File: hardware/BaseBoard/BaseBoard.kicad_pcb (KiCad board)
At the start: 2 copper layers, 81.5 x 109.2 mm, 91 parts, among them J1 I2C, J1-ESP1 ESP-1-L, J1-ESP2 ESP-1-L, J1-ESP3 ESP-1-L, J1-ESP4 ESP-1-L, J1-ESP5 ESP-1-L, J1-ESP6 ESP-1-L, J1-ESP7 ESP-1-L, J1-ESP8 ESP-1-L, J2 3V3P0_7, J2-ESP1 ESP-1-R, J2-ESP2 ESP-1-R, J2-ESP3 ESP-1-R, J2-ESP4 ESP-1-R, J2-ESP5 ESP-1-R, J2-ESP6 ESP-1-R, J2-ESP7 ESP-1-R, J2-ESP8 ESP-1-R, J3-BUS1 BUS1-IN1, J3-BUS2 BUS1-IN1, J3-BUS3 BUS1-IN1, J3-BUS4 BUS1-IN1, J3-BUS5 BUS1-IN1, J3-BUS6 BUS1-IN1, J3-BUS7 BUS1-IN1, J3-BUS8 BUS1-IN1, J4-BUS1 BUS1-IN2, J4-BUS2 BUS1-IN2, J4-BUS3 BUS1-IN2, J4-BUS4 BUS1-IN2, J4-BUS5 BUS1-IN2, J4-BUS6 BUS1-IN2, J4-BUS7 BUS1-IN2, J4-BUS8 BUS1-IN2, J5-BUS1 BUS1-OUT, J5-BUS2 BUS1-OUT, J5-BUS3 BUS1-OUT, J5-BUS4 BUS1-OUT, J5-BUS5 BUS1-OUT, J5-BUS6 BUS1-OUT, J5-BUS7 BUS1-OUT, J5-BUS8 BUS1-OUT, Q1-ESP1 2N3904, Q1-ESP2 2N3904, Q1-ESP3 2N3904, Q1-ESP4 2N3904, Q1-ESP5 2N3904, Q1-ESP6 2N3904, Q1-ESP7 2N3904, Q1-ESP8 2N3904, Q2-ESP1 AO3401A, Q2-ESP2 AO3401A, Q2-ESP3 AO3401A, Q2-ESP4 AO3401A, Q2-ESP5 AO3401A, Q2-ESP6 AO3401A, Q2-ESP7 AO3401A, Q2-ESP8 AO3401A, U1 AMS1117-3.3

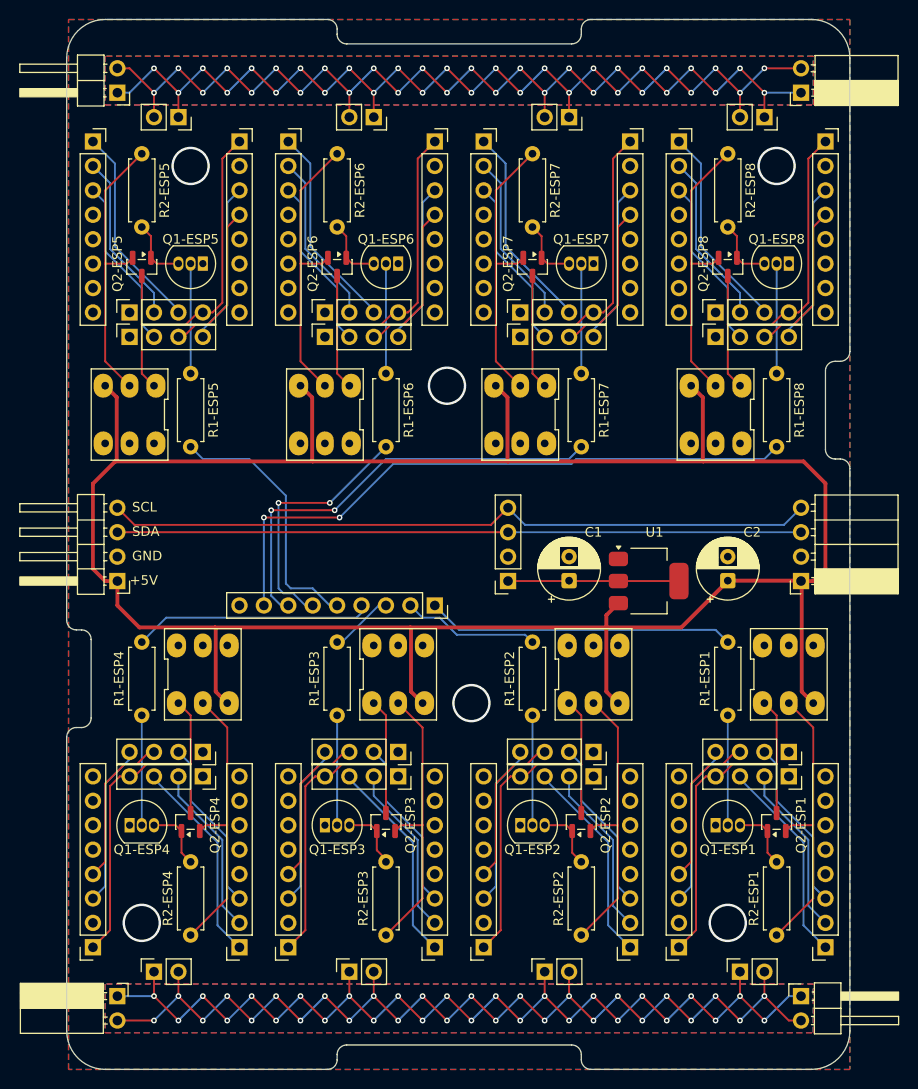
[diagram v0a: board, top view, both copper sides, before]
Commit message: Small optimizations.
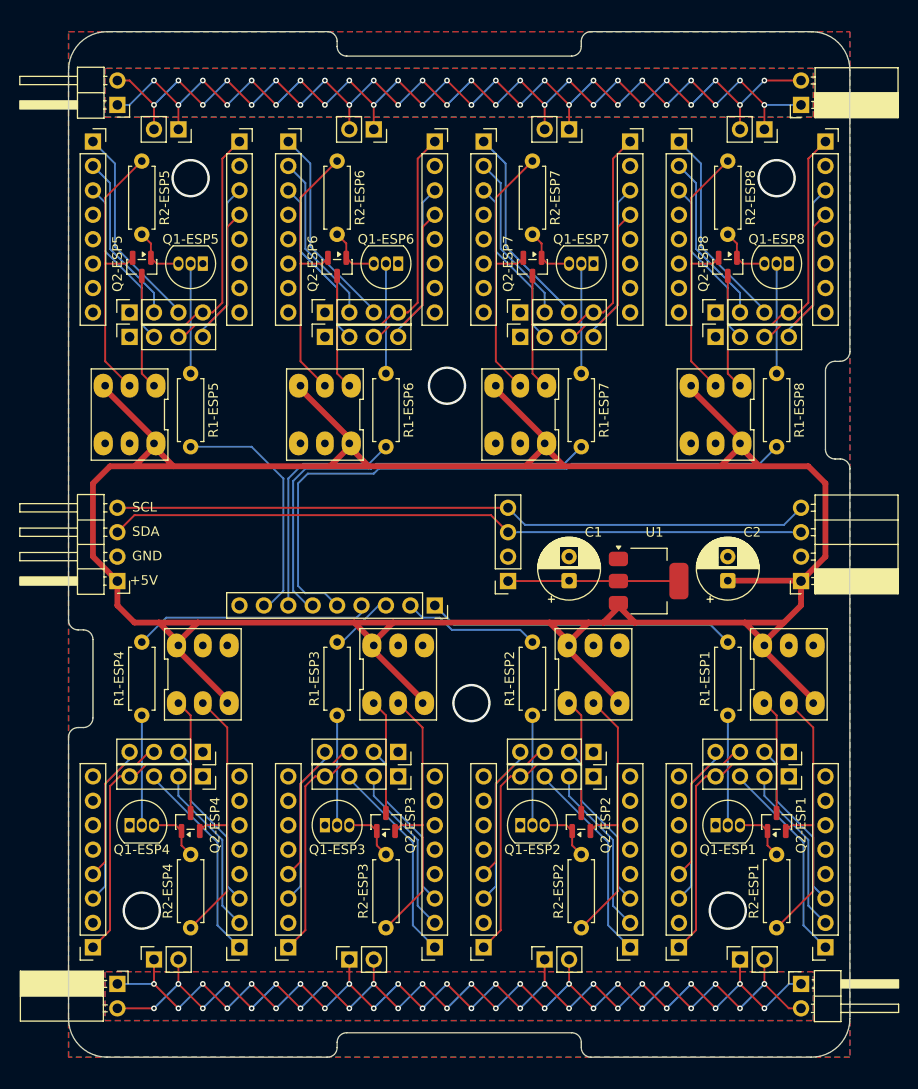
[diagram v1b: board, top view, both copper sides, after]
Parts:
- moved J5-BUS1 1.27 mm to (191.8, 115.6)
- moved J5-BUS2 1.27 mm to (171.4, 115.6)
- moved J5-BUS3 1.27 mm to (151.1, 115.6)
- moved J5-BUS4 1.27 mm to (130.8, 115.6)
- moved BUS_IN2 1.27 mm to (127.0, 26.7)
- moved BUS_OUT2 1.27 mm to (198.1, 26.7)
- moved J5-BUS5 1.27 mm to (133.3, 29.2)
- moved J5-BUS6 1.27 mm to (153.7, 29.2)
- moved J5-BUS7 1.27 mm to (174.0, 29.2)
- moved J5-BUS8 1.27 mm to (194.3, 29.2)
- moved BUS_IN1 1.27 mm to (198.1, 118.1)
- moved BUS_OUT1 1.27 mm to (127.0, 118.1)
- moved R2-ESP1 0.76 mm to (195.6, 112.3)
- moved R2-ESP2 0.76 mm to (175.3, 112.3)
- moved R2-ESP3 0.76 mm to (154.9, 112.3)
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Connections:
- J2 pad 5: SWPIN-ESP5 -> SWPIN-ESP8
- J2 pad 6: SWPIN-ESP6 -> SWPIN-ESP7
- J2 pad 7: SWPIN-ESP7 -> SWPIN-ESP6
- J2 pad 8: SWPIN-ESP8 -> SWPIN-ESP5
- SW-ESP1 pad 6: unconnected-(SW-ESP1-Pad6) -> +5V
- SW-ESP2 pad 6: unconnected-(SW-ESP2-Pad6) -> +5V
- SW-ESP3 pad 6: unconnected-(SW-ESP3-Pad6) -> +5V
- SW-ESP4 pad 6: unconnected-(SW-ESP4-Pad6) -> +5V
- SW-ESP5 pad 6: unconnected-(SW-ESP5-Pad6) -> +5V
- SW-ESP6 pad 6: unconnected-(SW-ESP6-Pad6) -> +5V
- SW-ESP7 pad 6: unconnected-(SW-ESP7-Pad6) -> +5V
- SW-ESP8 pad 6: unconnected-(SW-ESP8-Pad6) -> +5V
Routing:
- net +5V: track 253.7 -> 307.9 mm
- net SWPIN-ESP6: track 27.0 -> 24.7 mm, vias 2 -> 0
- net SWPIN-ESP5: track 27.4 -> 25.4 mm
- net I2C_SCL: track 74.1 -> 72.6 mm
- net I2C_SDA: track 71.1 -> 72.6 mm
- net SWPIN-ESP8: track 65.5 -> 66.9 mm, vias 2 -> 0
- net Net-(Q1-ESP1-C): track 6.85 -> 5.95 mm
- net Net-(Q2-ESP8-S): track 29.9 -> 29.1 mm
- net Net-(Q2-ESP7-S): track 29.9 -> 29.1 mm
- net Net-(Q2-ESP6-S): track 29.9 -> 29.1 mm
- net Net-(Q2-ESP5-S): track 29.9 -> 29.1 mm
- net Net-(Q2-ESP4-S): track 29.9 -> 29.1 mm
- net Net-(Q2-ESP3-S): track 29.9 -> 29.1 mm
- net Net-(Q2-ESP2-S): track 29.9 -> 29.1 mm
- net Net-(Q1-ESP8-C): track 6.71 -> 5.95 mm
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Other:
- board size 81.5 x 109.2 mm -> 81.3 x 106.7 mm
